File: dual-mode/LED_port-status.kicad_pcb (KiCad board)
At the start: 2 copper layers, 23.7 x 12.5 mm, 21 parts, among them P1 CONN_9

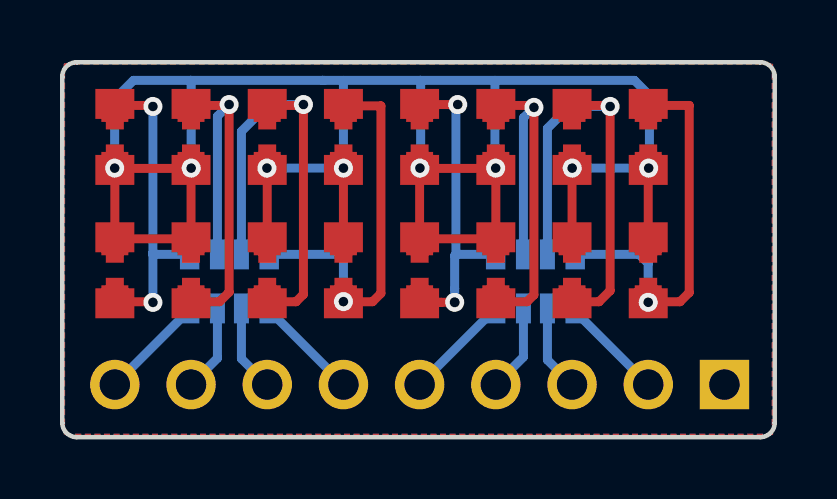
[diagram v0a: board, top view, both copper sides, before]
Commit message: Tiny layout tweek.
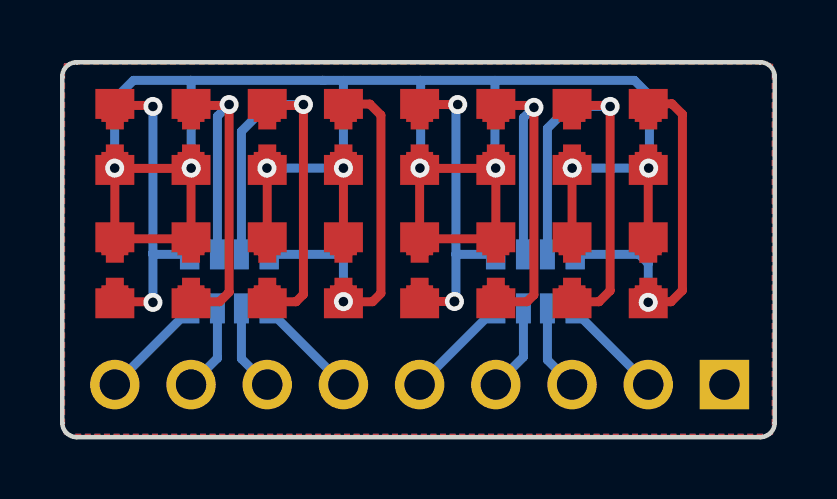
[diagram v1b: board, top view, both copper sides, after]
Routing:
- net Net-(D16-Pad1): track 13.0 -> 12.3 mm
